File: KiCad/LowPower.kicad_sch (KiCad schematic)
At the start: 42 parts, among them J1 Connector, J2 USB-C, J3 DC, Q1 RN1701, U1 ESP32-WROOM-32, U2 FT231XQ, U3 NX6020CAKS, U4 LMR16006+FB

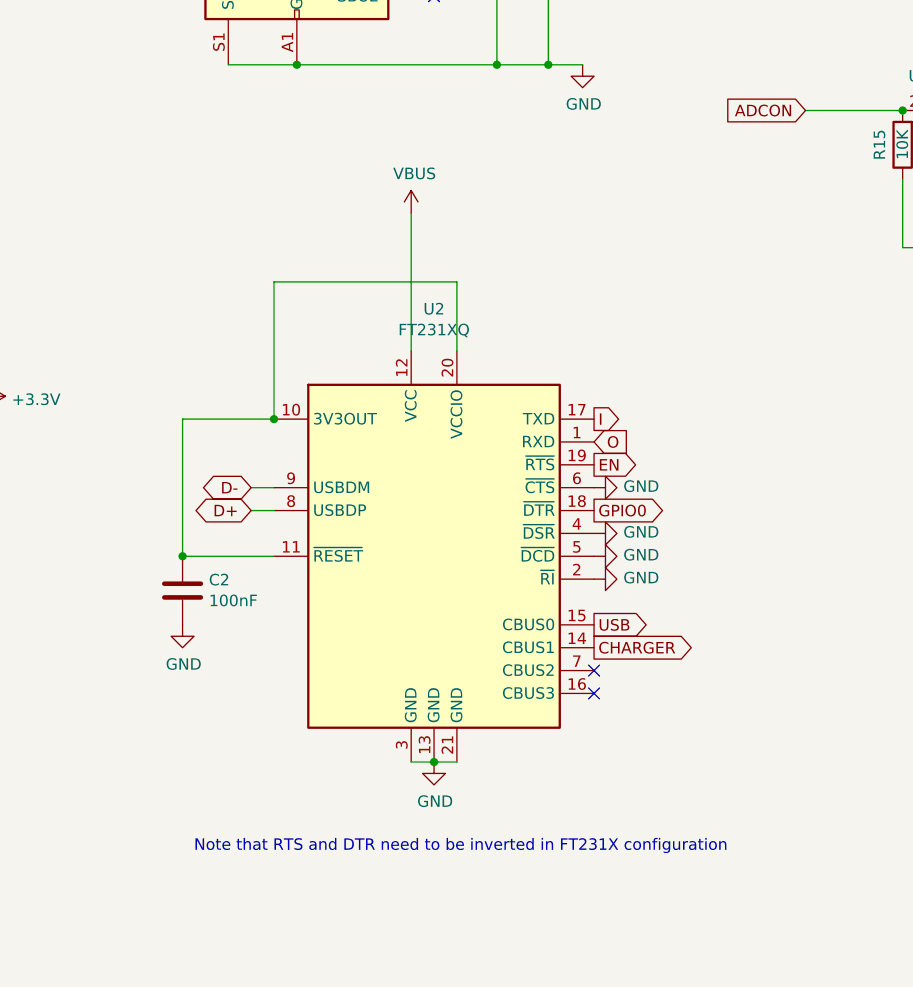
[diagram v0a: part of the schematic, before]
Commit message: Footprint update
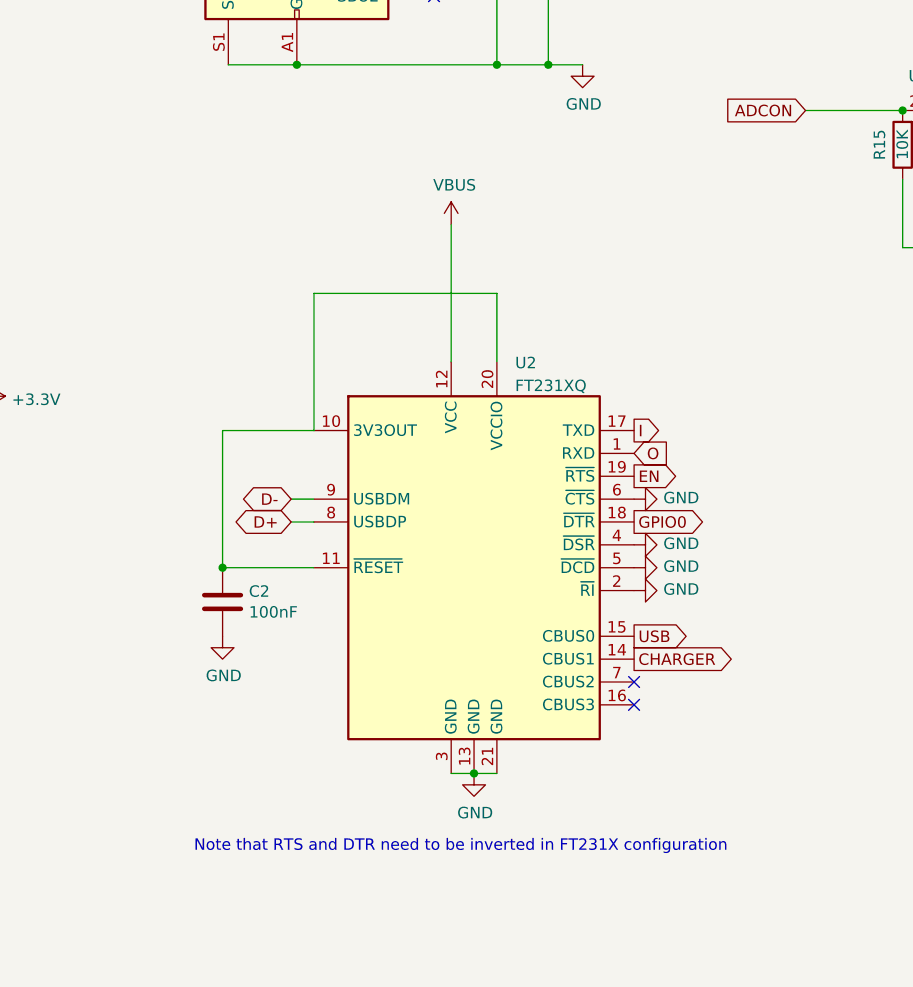
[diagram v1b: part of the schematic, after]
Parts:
- removed U2: FT231XQ, RevK:QFN-20-1EP_4x4mm_P0.5mm_EP2.5x2.5mm, symbol Interface_USB:FT231XQ
- added U2: FT231XQ, RevK:QFN-20-1EP_4x4mm_P0.5mm_EP2.5x2.5mm, symbol RevK:FT231XQ
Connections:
- net CHARGER: now also U2.14 (CBUS1)
- net D+: now also U2.8 (USBDP)
- net D-: now also U2.9 (USBDM)
- net EN: now also U2.19 (~{RTS})
- net GND: now also U2.13 (GND), U2.2 (~{RI}), U2.21 (GND), U2.3 (GND), U2.4 (~{DSR}), U2.5 (~{DCD}), U2.6 (~{CTS})
- net GPIO0: now also U2.18 (~{DTR})
- net I: now also U2.17 (TXD)
- net O: now also U2.1 (RXD)
- net USB: now also U2.15 (CBUS0)
- net VBUS: now also U2.12 (VCC)
- net at C2.1: now also U2.10 (3V3OUT), U2.11 (~{RESET}), U2.20 (VCCIO)
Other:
- moved on the sheet: C2
